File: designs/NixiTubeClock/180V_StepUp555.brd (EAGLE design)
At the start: 52.5 x 39 mm, 17 parts, among them IC1 IRF740SPBF, IC2 LM555D, T1 BC547

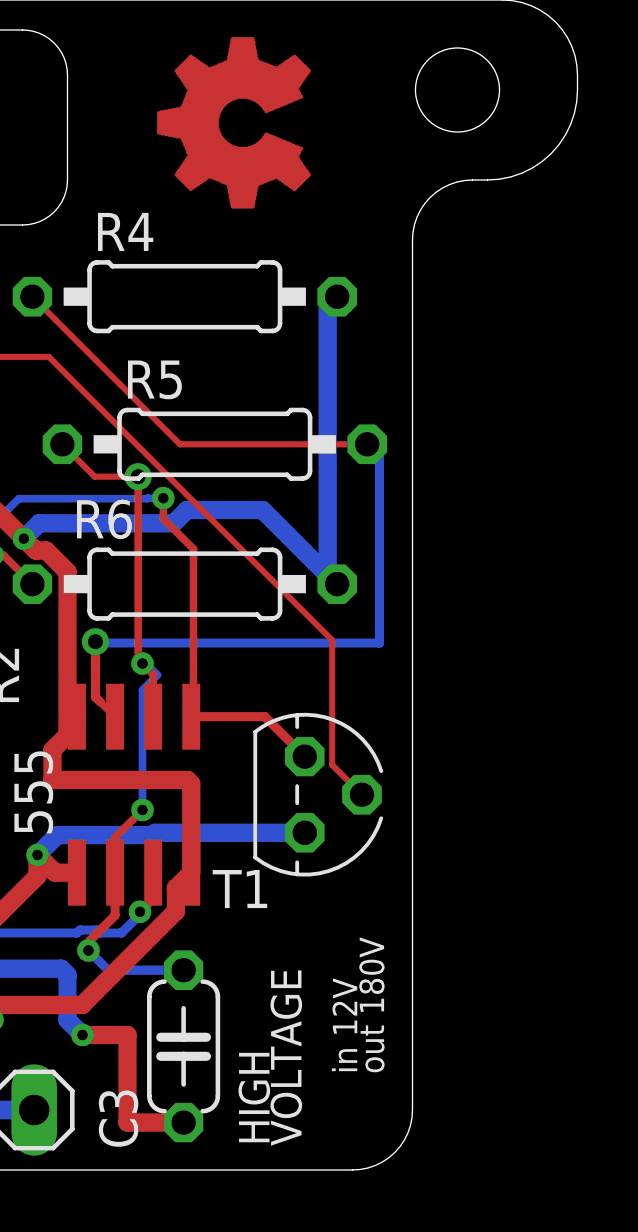
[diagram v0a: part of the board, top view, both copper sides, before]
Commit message: worked on brd layout NI-4
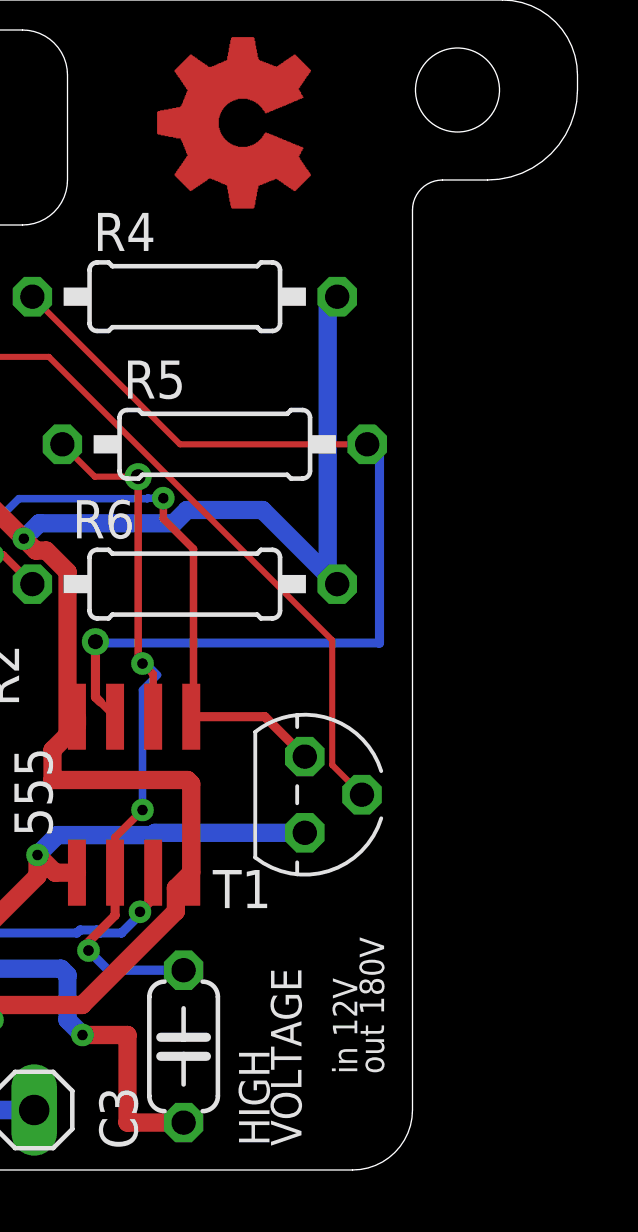
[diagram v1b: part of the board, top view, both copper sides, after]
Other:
- outline, holes or cut-outs redrawn
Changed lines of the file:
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@@
 <setting verticaltext="up"/>
 </settings>
-<grid distance="0.1" unitdist="mm" unit="mm" style="lines" multiple="1" display="yes" altdistance="5" altunitdist="mm" altunit="mm"/>
+<grid distance="0.5" unitdist="mm" unit="mm" style="lines" multiple="1" display="yes" altdistance="5" altunitdist="mm" altunit="mm"/>
 <layers>
 <layer number="1" name="Top" color="4" fill="1" visible="yes" active="yes"/>
@@
 <wire x1="11" y1="0" x2="50" y2="0" width="0" layer="20"/>
 <wire x1="50" y1="0" x2="52" y2="2" width="0" layer="20" curve="90"/>
-<wire x1="54.5" y1="33" x2="54" y2="33" width="0" layer="20"/>
-<wire x1="54" y1="33" x2="52" y2="31" width="0" layer="20" curve="90"/>
-<wire x1="52" y1="31" x2="52" y2="2" width="0" layer="20"/>
+<wire x1="54.5" y1="33" x2="53" y2="33" width="0" layer="20"/>
+<wire x1="53" y1="33" x2="52" y2="32" width="0" layer="20" curve="90"/>
+<wire x1="52" y1="32" x2="52" y2="2" width="0" layer="20"/>
 <wire x1="40.5" y1="33" x2="40.5" y2="36.5" width="0" layer="20"/>
 <wire x1="40.5" y1="36.5" x2="39" y2="38" width="0" layer="20" curve="90"/>
